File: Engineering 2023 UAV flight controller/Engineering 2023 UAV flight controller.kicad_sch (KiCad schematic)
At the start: 12 parts

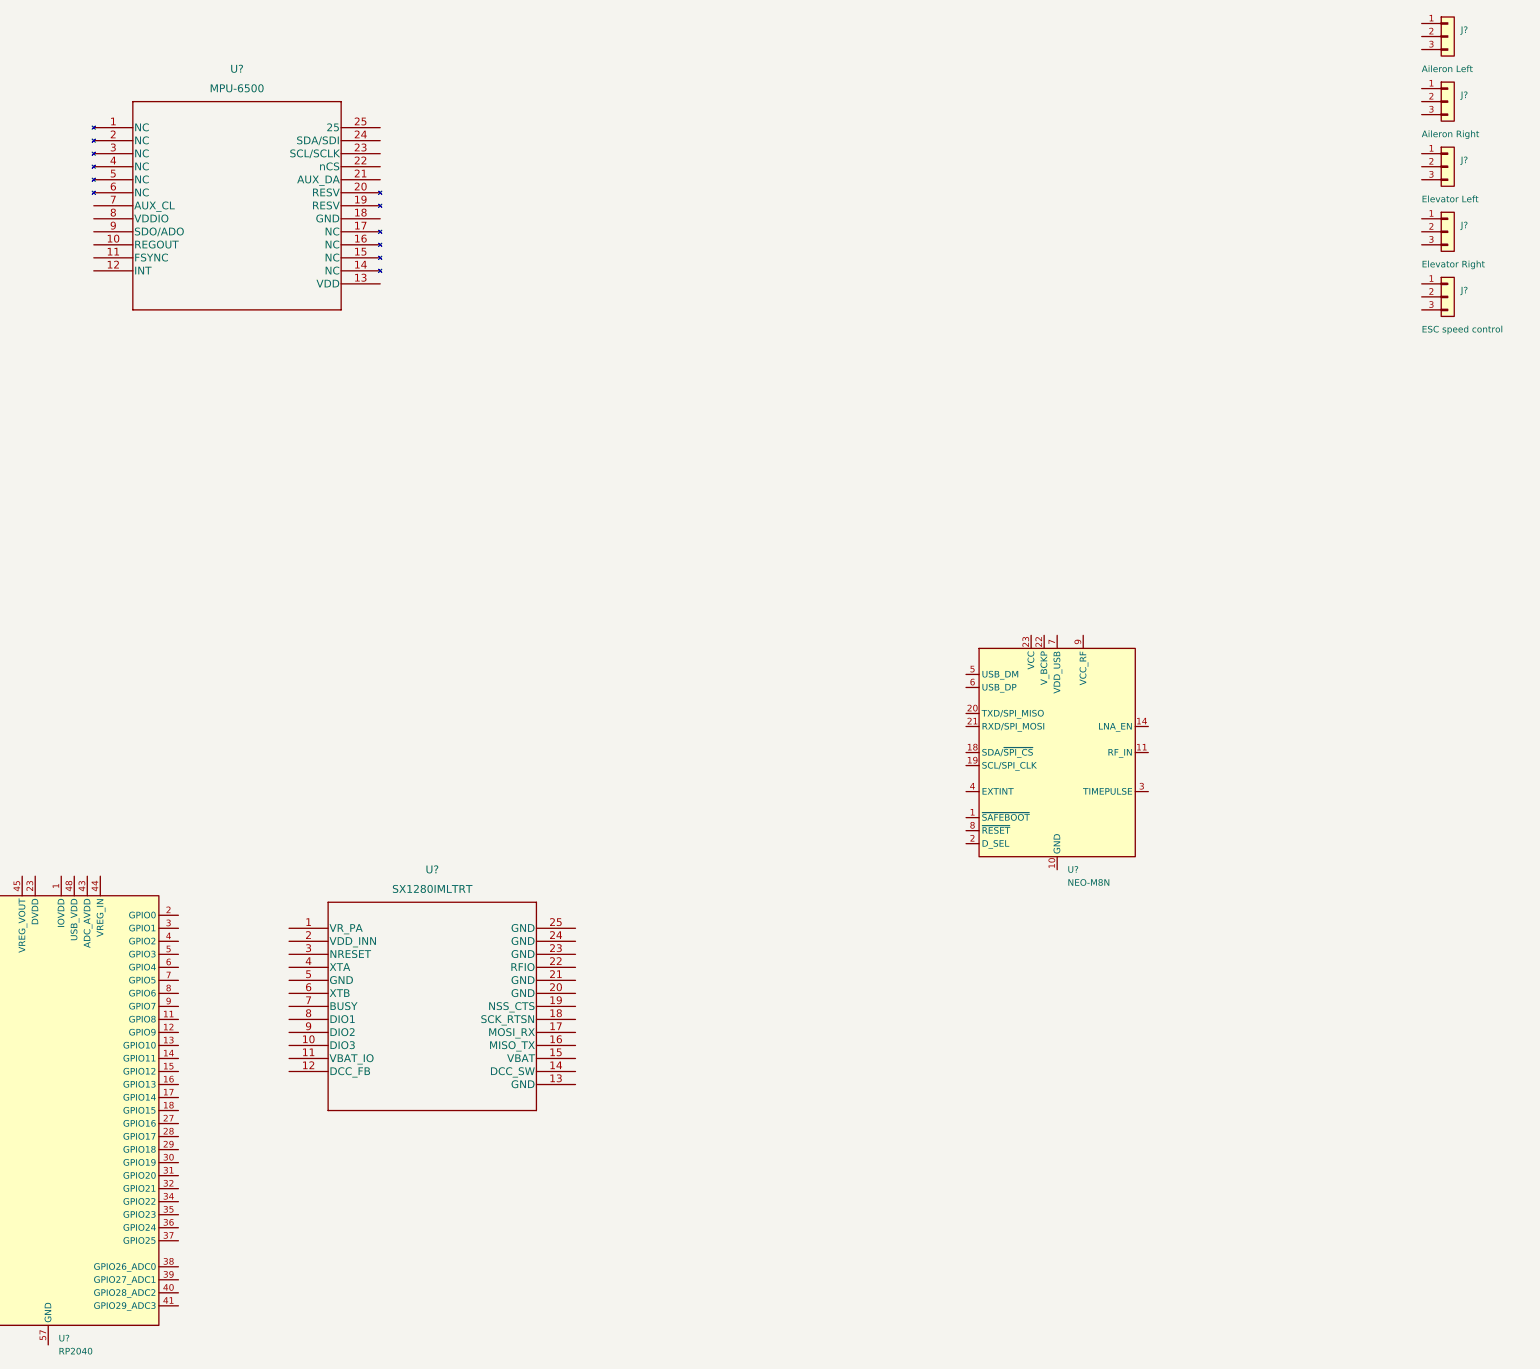
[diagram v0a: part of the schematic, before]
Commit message: dont remember changes, were last night
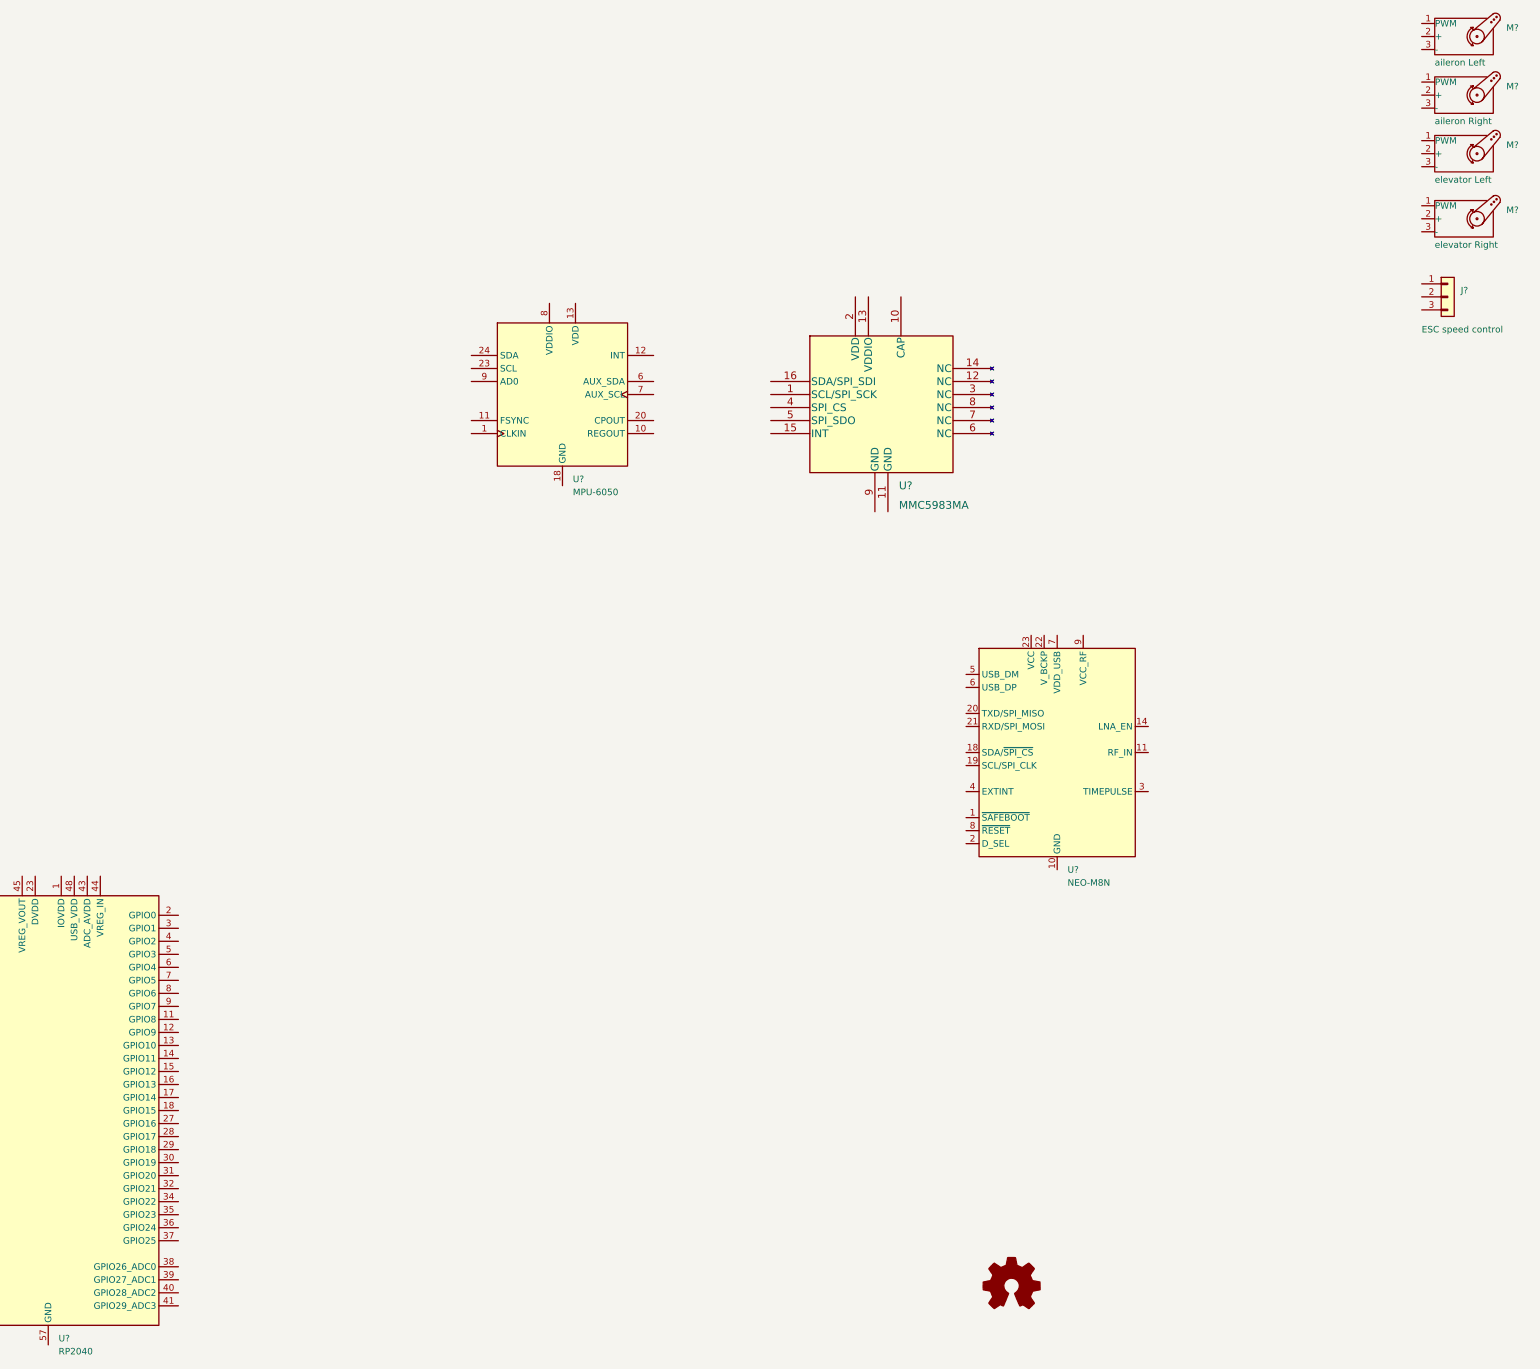
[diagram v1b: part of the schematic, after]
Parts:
- removed J?: Aileron Right, symbol Connector_Generic:Conn_01x03
- removed J?: Elevator Left, symbol Connector_Generic:Conn_01x03
- removed J?: Elevator Right, symbol Connector_Generic:Conn_01x03
- removed J?: Aileron Left, symbol Connector_Generic:Conn_01x03
- removed U?: MPU-6500, QFN24_3X3X0P9_IVS, symbol MPU-6500:MPU-6500
- removed U?: SX1280IMLTRT, QFN24_4X4_SEM, symbol SX1280:SX1280IMLTRT
- added M?: elevator Left, symbol Motor:Motor_Servo
- added M?: elevator Right, symbol Motor:Motor_Servo
- added M?: aileron Right, symbol Motor:Motor_Servo
- added M?: aileron Left, symbol Motor:Motor_Servo
- added U?: MMC5983MA, MMC5983MA_MEM, symbol MMC5983MA:MMC5983MA
- added U?: MPU-6050, Sensor_Motion:InvenSense_QFN-24_4x4mm_P0.5mm, symbol Sensor_Motion:MPU-6050
- J?: footprint (none) -> Connector_USB:USB_C_Receptacle_JAE_DX07S016JA1R1500

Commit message: some small updates
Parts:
- M?: value elevator Left -> Elevator Left
- M?: value elevator Right -> Elevator Right
- M?: value aileron Right -> Aileron Right
- M?: value aileron Left -> Aileron Left
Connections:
- net Elevator Left PWM: now reaches M?.1 (PWM)
- net Elevator Right PWM: now reaches M?.1 (PWM)
- net Aileron Right PWM: now reaches M?.1 (PWM)
- net Aileron Left PWM: now reaches M?.1 (PWM)
- net ESC PWM: now reaches J?.1 (Pin_1)
- net ESC positive rail: now reaches J?.2 (Pin_2)
- net ESC negitive rail: now reaches J?.3 (Pin_3)
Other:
- moved on the sheet: J?, U?
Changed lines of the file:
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@@
 (kicad_sch (version 20211123) (generator eeschema)
   (paper "A3")
+  (wire (pts (xy 368.3 50.8) (xy 388.62 50.8))
+    (stroke (width 0) (type default) (color 0 0 0 0))
+  )
+  (wire (pts (xy 368.3 63.5) (xy 388.62 63.5))
+    (stroke (width 0) (type default) (color 0 0 0 0))
+  )
+  (wire (pts (xy 368.3 26.67) (xy 388.62 26.67))
+    (stroke (width 0) (type default) (color 0 0 0 0))
+  )
+  (wire (pts (xy 368.3 38.1) (xy 388.62 38.1))
+    (stroke (width 0) (type default) (color 0 0 0 0))
+  )
+  (wire (pts (xy 368.3 66.04) (xy 388.62 66.04))
+    (stroke (width 0) (type default) (color 0 0 0 0))
+  )
+  (wire (pts (xy 368.3 15.24) (xy 388.62 15.24))
+    (stroke (width 0) (type default) (color 0 0 0 0))
+  )
+  (wire (pts (xy 368.3 68.58) (xy 388.62 68.58))
+    (stroke (width 0) (type default) (color 0 0 0 0))
+  )
+  (label "Elevator Right PWM" (at 368.3 50.8 0)
+    (effects (font (size 1.27 1.27)) (justify left bottom))
+  )
+  (label "Aileron Left PWM" (at 368.3 15.24 0)
+    (effects (font (size 1.27 1.27)) (justify left bottom))
+  )
+  (label "ESC positive rail" (at 368.3 66.04 0)
+    (effects (font (size 1.27 1.27)) (justify left bottom))
+  )
+  (label "Elevator Left PWM" (at 368.3 38.1 0)
+    (effects (font (size 1.27 1.27)) (justify left bottom))
+  )
+  (label "ESC PWM" (at 368.3 63.5 0)
+    (effects (font (size 1.27 1.27)) (justify left bottom))
+  )
+  (label "ESC negitive rail" (at 368.3 68.58 0)
+    (effects (font (size 1.27 1.27)) (justify left bottom))
+  )
+  (label "Aileron Right PWM" (at 368.3 26.67 0)
+    (effects (font (size 1.27 1.27)) (justify left bottom))
+  )
   (symbol (lib_id "Motor:Motor_Servo") (at 396.24 40.64 0) (unit 1)
     (in_bom yes) (on_board yes)
@@
       (effects (font (size 1.27 1.27)) (justify left))
     )
-    (property "Value" "elevator Left" (id 1) (at 391.16 45.72 0)
+    (property "Value" "Elevator Left" (id 1) (at 388.62 45.72 0)
       (effects (font (size 1.27 1.27)) (justify left))
     )
@@
       (effects (font (size 1.27 1.27)) (justify left))
     )
-    (property "Value" "elevator Right" (id 1) (at 391.16 58.42 0)
+    (property "Value" "Elevator Right" (id 1) (at 388.62 58.42 0)
       (effects (font (size 1.27 1.27)) (justify left))
     )
@@
     (pin "S1")
   )
-  (symbol (lib_id "Sensor_Motion:MPU-6050") (at 220.98 87.63 0) (unit 1)
-    (in_bom yes) (on_board yes) (fields_autoplaced)
-    (property "Reference" "U?" (id 0) (at 222.9994 104.14 0)
-      (effects (font (size 1.27 1.27)) (justify left))
-    )
-    (property "Value" "MPU-6050" (id 1) (at 222.9994 106.68 0)
-      (effects (font (size 1.27 1.27)) (justify left))
-    )
-    (property "Footprint" "Sensor_Motion:InvenSense_QFN-24_4x4mm_P0.5mm" (id 2) (at 220.98 107.95 0)
-      (effects (font (size 1.27 1.27)) hide)
-    )
-    (property "Datasheet" "https://store.invensense.com/datasheets/invensense/MPU-6050_DataSheet_V3%204.pdf" (id 3) (at 220.98 91.44 0)
+  (symbol (lib_id "Sensor_Motion:MPU-6050") (at 229.87 88.9 0) (unit 1)
+    (in_bom yes) (on_board yes) (fields_autoplaced)
+    (property "Reference" "U?" (id 0) (at 231.8894 105.41 0)
+      (effects (font (size 1.27 1.27)) (justify left))
+    )
+    (property "Value" "MPU-6050" (id 1) (at 231.8894 107.95 0)
+      (effects (font (size 1.27 1.27)) (justify left))
+    )
+    (property "Footprint" "Sensor_Motion:InvenSense_QFN-24_4x4mm_P0.5mm" (id 2) (at 229.87 109.22 0)
+      (effects (font (size 1.27 1.27)) hide)
+    )
+    (property "Datasheet" "https://store.invensense.com/datasheets/invensense/MPU-6050_DataSheet_V3%204.pdf" (id 3) (at 229.87 92.71 0)
       (effects (font (size 1.27 1.27)) hide)
     )
@@
       (effects (font (size 1.27 1.27)) (justify left))
     )
-    (property "Value" "aileron Right" (id 1) (at 391.16 34.29 0)
+    (property "Value" "Aileron Right" (id 1) (at 388.62 34.29 0)
       (effects (font (size 1.27 1.27)) (justify left))
     )
@@
     (pin "3")
   )
-  (symbol (lib_id "Connector:Micro_SD_Card") (at 34.29 104.14 0) (mirror y) (unit 1)
-    (in_bom yes) (on_board yes) (fields_autoplaced)
-    (property "Reference" "J?" (id 0) (at 33.655 85.09 0))
-    (property "Value" "Micro_SD_Card" (id 1) (at 33.655 87.63 0))
-    (property "Footprint" "" (id 2) (at 5.08 96.52 0)
-      (effects (font (size 1.27 1.27)) hide)
-    )
-    (property "Datasheet" "http://katalog.we-online.de/em/datasheet/693072010801.pdf" (id 3) (at 34.29 104.14 0)
+  (symbol (lib_id "Connector:Micro_SD_Card") (at 247.65 144.78 0) (mirror x) (unit 1)
+    (in_bom yes) (on_board yes) (fields_autoplaced)
+    (property "Reference" "J?" (id 0) (at 248.285 123.19 0))
+    (property "Value" "Micro_SD_Card" (id 1) (at 248.285 125.73 0))
+    (property "Footprint" "" (id 2) (at 276.86 152.4 0)
+      (effects (font (size 1.27 1.27)) hide)
+    )
+    (property "Datasheet" "http://katalog.we-online.de/em/datasheet/693072010801.pdf" (id 3) (at 247.65 144.78 0)
       (effects (font (size 1.27 1.27)) hide)
     )
@@
       (effects (font (size 1.27 1.27)) (justify left))
     )
-    (property "Value" "aileron Left" (id 1) (at 391.16 22.86 0)
+    (property "Value" "Aileron Left" (id 1) (at 388.62 22.86 0)
       (effects (font (size 1.27 1.27)) (justify left))
     )
@@
     (pin "3")
   )
-  (symbol (lib_id "RF_GPS:NEO-M8N") (at 317.5 157.48 0) (unit 1)
-    (in_bom yes) (on_board yes) (fields_autoplaced)
-    (property "Reference" "U?" (id 0) (at 319.5194 180.34 0)
-      (effects (font (size 1.27 1.27)) (justify left))
-    )
-    (property "Value" "NEO-M8N" (id 1) (at 319.5194 182.88 0)
-      (effects (font (size 1.27 1.27)) (justify left))
-    )
-    (property "Footprint" "RF_GPS:ublox_NEO" (id 2) (at 327.66 179.07 0)
-      (effects (font (size 1.27 1.27)) hide)
-    )
-    (property "Datasheet" "https://www.u-blox.com/sites/default/files/NEO-M8-FW3_DataSheet_%28UBX-15031086%29.pdf" (id 3) (at 317.5 157.48 0)
+  (symbol (lib_id "RF_GPS:NEO-M8N") (at 365.76 205.74 0) (unit 1)
+    (in_bom yes) (on_board yes) (fields_autoplaced)
+    (property "Reference" "U?" (id 0) (at 367.7794 228.6 0)
+      (effects (font (size 1.27 1.27)) (justify left))
+    )
+    (property "Value" "NEO-M8N" (id 1) (at 367.7794 231.14 0)
+      (effects (font (size 1.27 1.27)) (justify left))
+    )
+    (property "Footprint" "RF_GPS:ublox_NEO" (id 2) (at 375.92 227.33 0)
+      (effects (font (size 1.27 1.27)) hide)
+    )
+    (property "Datasheet" "https://www.u-blox.com/sites/default/files/NEO-M8-FW3_DataSheet_%28UBX-15031086%29.pdf" (id 3) (at 365.76 205.74 0)
       (effects (font (size 1.27 1.27)) hide)
     )
@@
     (pin "9")
   )
-  (symbol (lib_id "Connector_Generic:Conn_01x03") (at 393.7 68.58 0) (unit 1)
+  (symbol (lib_id "Connector_Generic:Conn_01x03") (at 393.7 66.04 0) (unit 1)
     (in_bom yes) (on_board yes)
-    (property "Reference" "J?" (id 0) (at 396.24 67.3099 0)
-      (effects (font (size 1.27 1.27)) (justify left))
-    )
-    (property "Value" "ESC speed control" (id 1) (at 388.62 74.93 0)
-      (effects (font (size 1.27 1.27)) (justify left))
-    )
-    (property "Footprint" "" (id 2) (at 393.7 68.58 0)
-      (effects (font (size 1.27 1.27)) hide)
-    )
-    (property "Datasheet" "~" (id 3) (at 393.7 68.58 0)
+    (property "Reference" "J?" (id 0) (at 396.24 64.7699 0)
+      (effects (font (size 1.27 1.27)) (justify left))
+    )
+    (property "Value" "ESC speed control" (id 1) (at 388.62 72.39 0)
+      (effects (font (size 1.27 1.27)) (justify left))
+    )
+    (property "Footprint" "" (id 2) (at 393.7 66.04 0)
+      (effects (font (size 1.27 1.27)) hide)
+    )
+    (property "Datasheet" "~" (id 3) (at 393.7 66.04 0)
       (effects (font (size 1.27 1.27)) hide)
     )
@@
     )
     (path "/10ec48c8-c7b5-43a4-bb63-38ddcdfa745e"
-      (reference "M?") (unit 1) (value "elevator Left") (footprint "")
+      (reference "M?") (unit 1) (value "Elevator Left") (footprint "")
     )
     (path "/4e2503e3-7522-4959-b540-6c7684261f30"
-      (reference "M?") (unit 1) (value "elevator Right") (footprint "")
+      (reference "M?") (unit 1) (value "Elevator Right") (footprint "")
     )
     (path "/a5803e7c-8b9f-45cb-9ce9-ade452865f1b"
-      (reference "M?") (unit 1) (value "aileron Right") (footprint "")
+      (reference "M?") (unit 1) (value "Aileron Right") (footprint "")
     )
     (path "/d40a1cc5-fbc2-4c1e-9349-e721bb07408e"
-      (reference "M?") (unit 1) (value "aileron Left") (footprint "")
+      (reference "M?") (unit 1) (value "Aileron Left") (footprint "")
     )
     (path "/357beecd-919b-401e-b840-f3b5be37c3a3"
